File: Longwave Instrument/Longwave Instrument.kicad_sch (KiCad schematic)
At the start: 39 parts, among them U13 ADR5045B, U8 ADR510, U9 ADR5043B

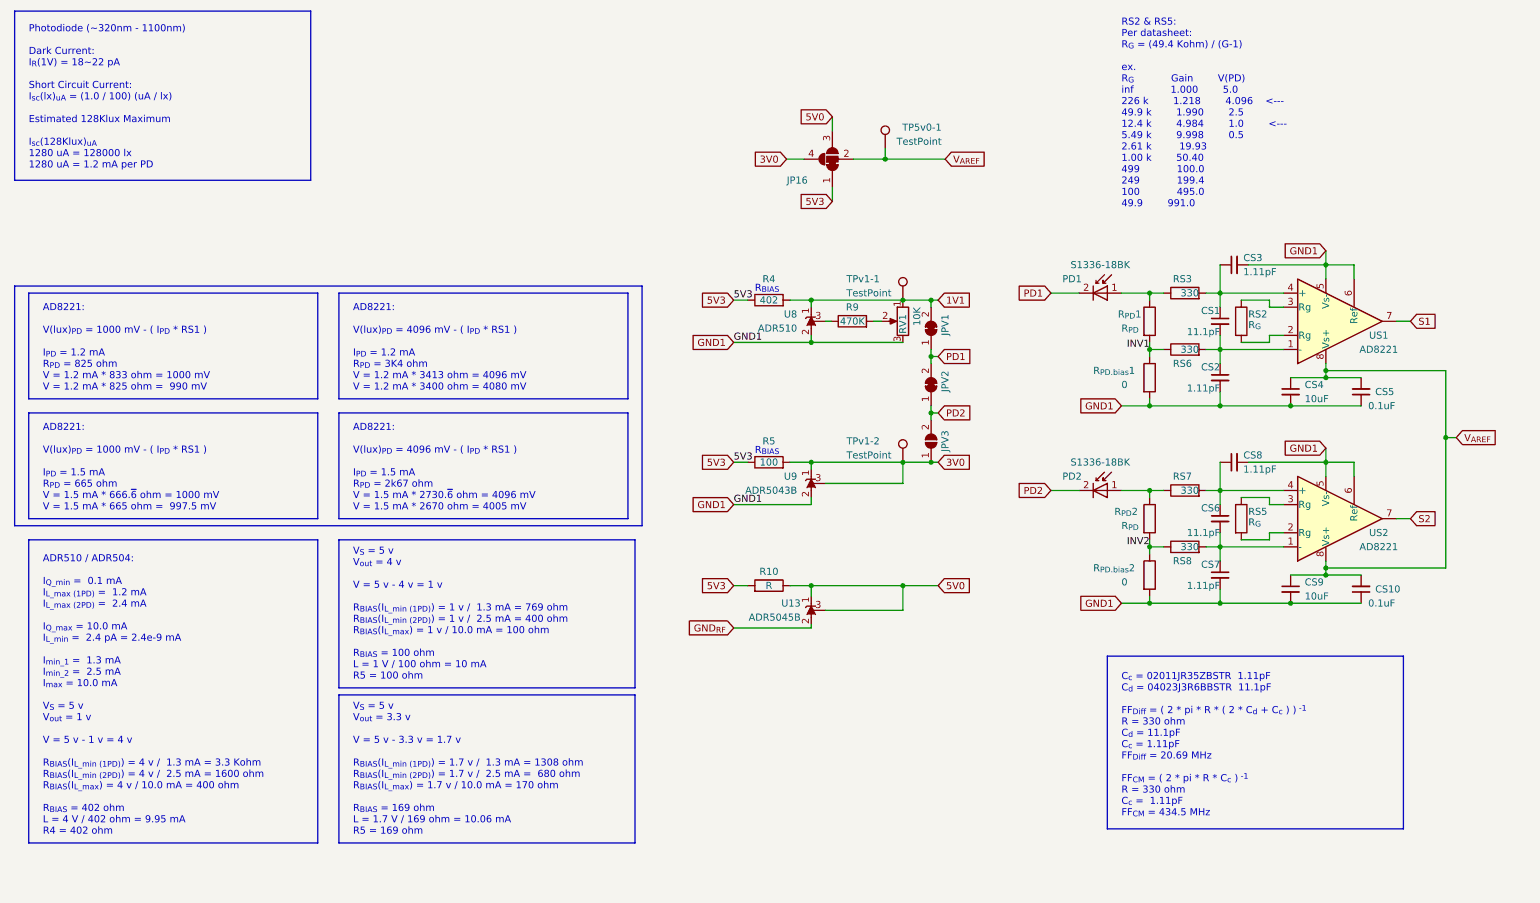
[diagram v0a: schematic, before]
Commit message: SpectDrone Development
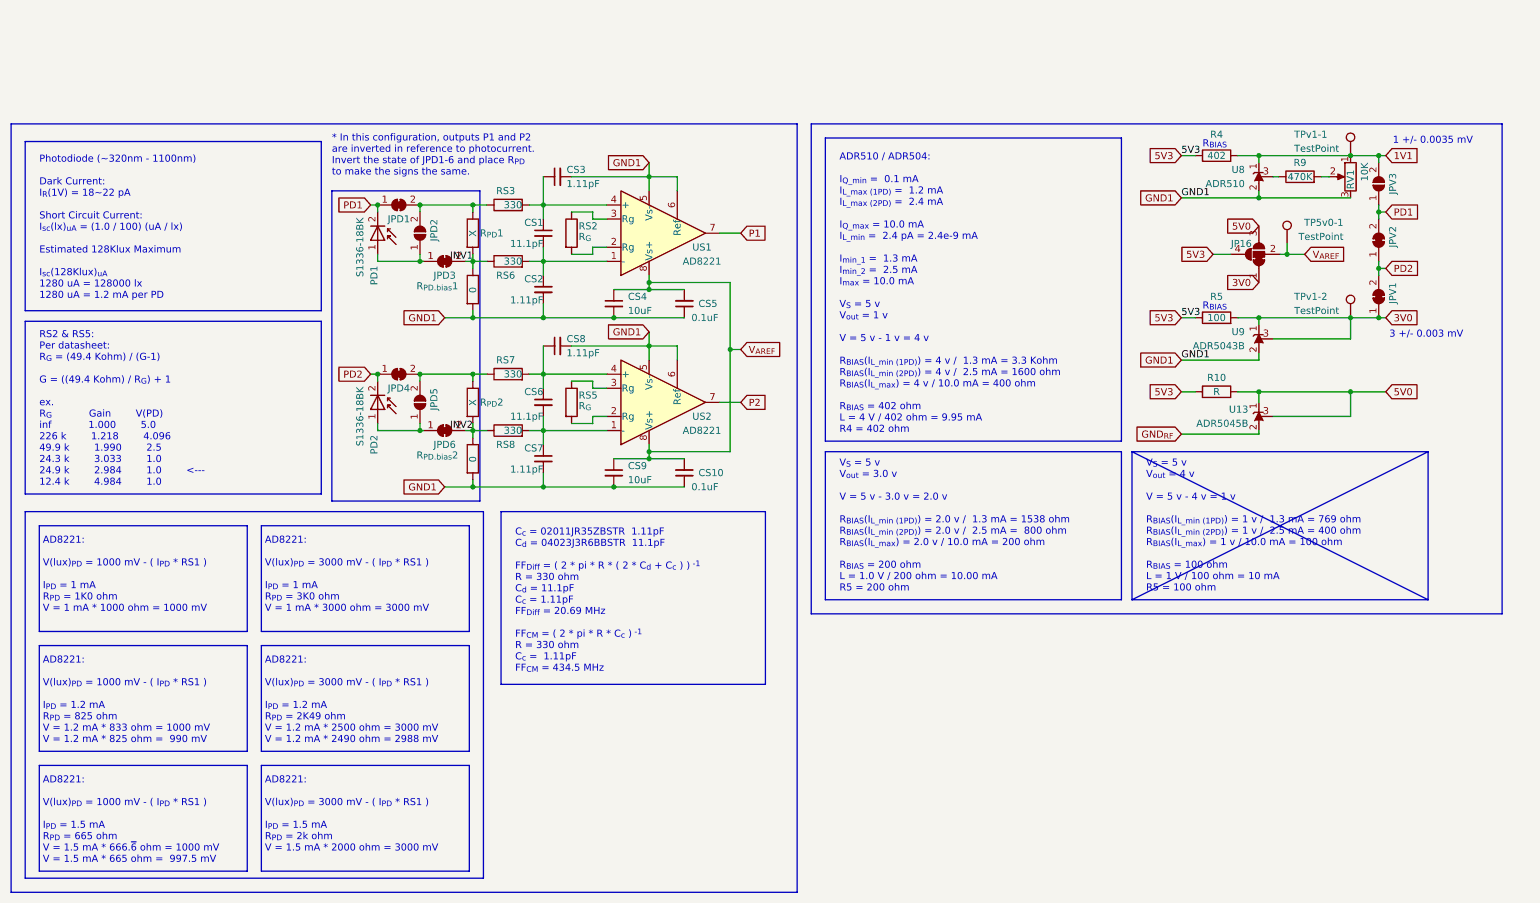
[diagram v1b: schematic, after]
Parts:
- added JPD1, JPD3, JPD4, JPD6: SolderJumper_2_Bridged, Jumper:SolderJumper-2_P1.3mm_Bridged_RoundedPad1.0x1.5mm, symbol Jumper:SolderJumper_2_Bridged
- added JPD2, JPD5: SolderJumper_2_Open, Jumper:SolderJumper-2_P1.3mm_Open_RoundedPad1.0x1.5mm, symbol Jumper:SolderJumper_2_Open
- R_{PD}1, R_{PD}2: value R_{PD} -> X
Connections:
- net 1V1: now also JPV3.2 (B); no longer JPV1.2 (B)
- net 3V0: now also JP16.1 (A), JPV1.1 (A); no longer JP16.4 (B), JPV3.1 (A)
- net 5V3: now also JP16.4 (B); no longer JP16.1 (A)
- net INV1: now also JPD3.2 (B)
- net INV2: now also JPD6.2 (B)
- net PD1: now also JPV3.1 (A), JPD1.1 (A); no longer JPV1.1 (A)
- net PD2: now also JPV1.2 (B), JPD4.1 (A); no longer JPV3.2 (B)
- net at RS7.1, R_{PD}2.1: now also JPD4.2 (B), JPD5.2 (B); no longer PD2.1 (A)
- net at RS3.1, R_{PD}1.1: now also JPD1.2 (B), JPD2.2 (B); no longer PD1.1 (A)
- net S1 renamed P1
- net S2 renamed P2
- new net: JPD5.1 (A), JPD6.1 (A), PD2.1 (A)
- new net: JPD2.1 (A), JPD3.1 (A), PD1.1 (A)
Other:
- note added: "* In this configuration, outputs P1 and P2 are inverted in reference to photocurrent. Invert the state of JPD1-6 and place R_{PD} to make the signs the same."
- note added: "1 +/- 0.0035 mV"
- note added: "3 +/- 0.003 mV"
- note added: "AD8221: V(lux)_{PD} = 1000 mV - ( I_{PD} * RS1 ) I_{PD} = 1 mA R_{PD} = 1K0 ohm V = 1 mA * 1000 ohm = 1000 mV"
- note added: "AD8221: V(lux)_{PD} = 3000 mV - ( I_{PD} * RS1 ) I_{PD} = 1 mA R_{PD} = 3K0 ohm V = 1 mA * 3000 ohm = 3000 mV"
- note added: "AD8221: V(lux)_{PD} = 3000 mV - ( I_{PD} * RS1 ) I_{PD} = 1.2 mA R_{PD} = 2K49 ohm V = 1.2 mA * 2500 ohm = 3000 mV V = 1.2 mA * 2490 ohm = 2988 mV"
- note added: "AD8221: V(lux)_{PD} = 3000 mV - ( I_{PD} * RS1 ) I_{PD} = 1.5 mA R_{PD} = 2k ohm V = 1.5 mA * 2000 ohm = 3000 mV"
- note added: "RS2 & RS5: Per datasheet: R_{G} = (49.4 Kohm) / (G-1) G = ((49.4 Kohm) / R_{G}) + 1 ex. R_{G} Gain V(PD) inf 1.000 5.0 226 k 1.218 4.096 49.9 k 1.990 2.5 24.3 k 3.033 1.0 24.9 k 2.984 1.0 <--- 12.4 k 4.984 1.0"
- note added: "V_{S} = 5 v V_{out} = 3.0 v V = 5 v - 3.0 v = 2.0 v R_{BIAS}(I_{L_min (1PD)}) = 2.0 v / 1.3 mA = 1538 ohm R_{BIAS}(I_{L_min (2PD)}) = 2.0 v / 2.5 mA = 800 ohm R_{BIAS}(I_{L_max}) = 2.0 v / 10.0 mA = 200 ohm R_{BIAS} = 200 ohm L = 1.0 V / 200 ohm = 10.00 mA R5 = 200 ohm"
- note removed: "AD8221: V(lux)_{PD} = 4096 mV - ( I_{PD} * RS1 ) I_{PD} = 1.2 mA R_{PD} = 3K4 ohm V = 1.2 mA * 3413 ohm = 4096 mV V = 1.2 mA * 3400 ohm = 4080 mV"
- note removed: "AD8221: V(lux)_{PD} = 4096 mV - ( I_{PD} * RS1 ) I_{PD} = 1.5 mA R_{PD} = 2k67 ohm V = 1.5 mA * 2730.~{6} ohm = 4096 mV V = 1.5 mA * 2670 ohm = 4005 mV"
- note removed: "RS2 & RS5: Per datasheet: R_{G} = (49.4 Kohm) / (G-1) ex. R_{G} Gain V(PD) inf 1.000 5.0 226 k 1.218 4.096 <--- 49.9 k 1.990 2.5 12.4 k 4.984 1.0 <--- 5.49 k 9.998 0.5 2.61 k 19.93 1.00 k 50.40 499 100.0 249 199.4 100 495.0 49.9 991.0"
- note removed: "V_{S} = 5 v V_{out} = 3.3 v V = 5 v - 3.3 v = 1.7 v R_{BIAS}(I_{L_min (1PD)}) = 1.7 v / 1.3 mA = 1308 ohm R_{BIAS}(I_{L_min (2PD)}) = 1.7 v / 2.5 mA = 680 ohm R_{BIAS}(I_{L_max}) = 1.7 v / 10.0 mA = 170 ohm R_{BIAS} = 169 ohm L = 1.7 V / 169 ohm = 10.06 mA R5 = 169 ohm"
- moved on the sheet: CS1, CS10, CS2, CS3, CS4, CS5, CS6, CS7, CS8, CS9, JP16, JPV1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
